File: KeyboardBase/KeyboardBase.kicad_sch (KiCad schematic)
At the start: 2 parts, among them J101 Conn_01x07, U101 74HC00

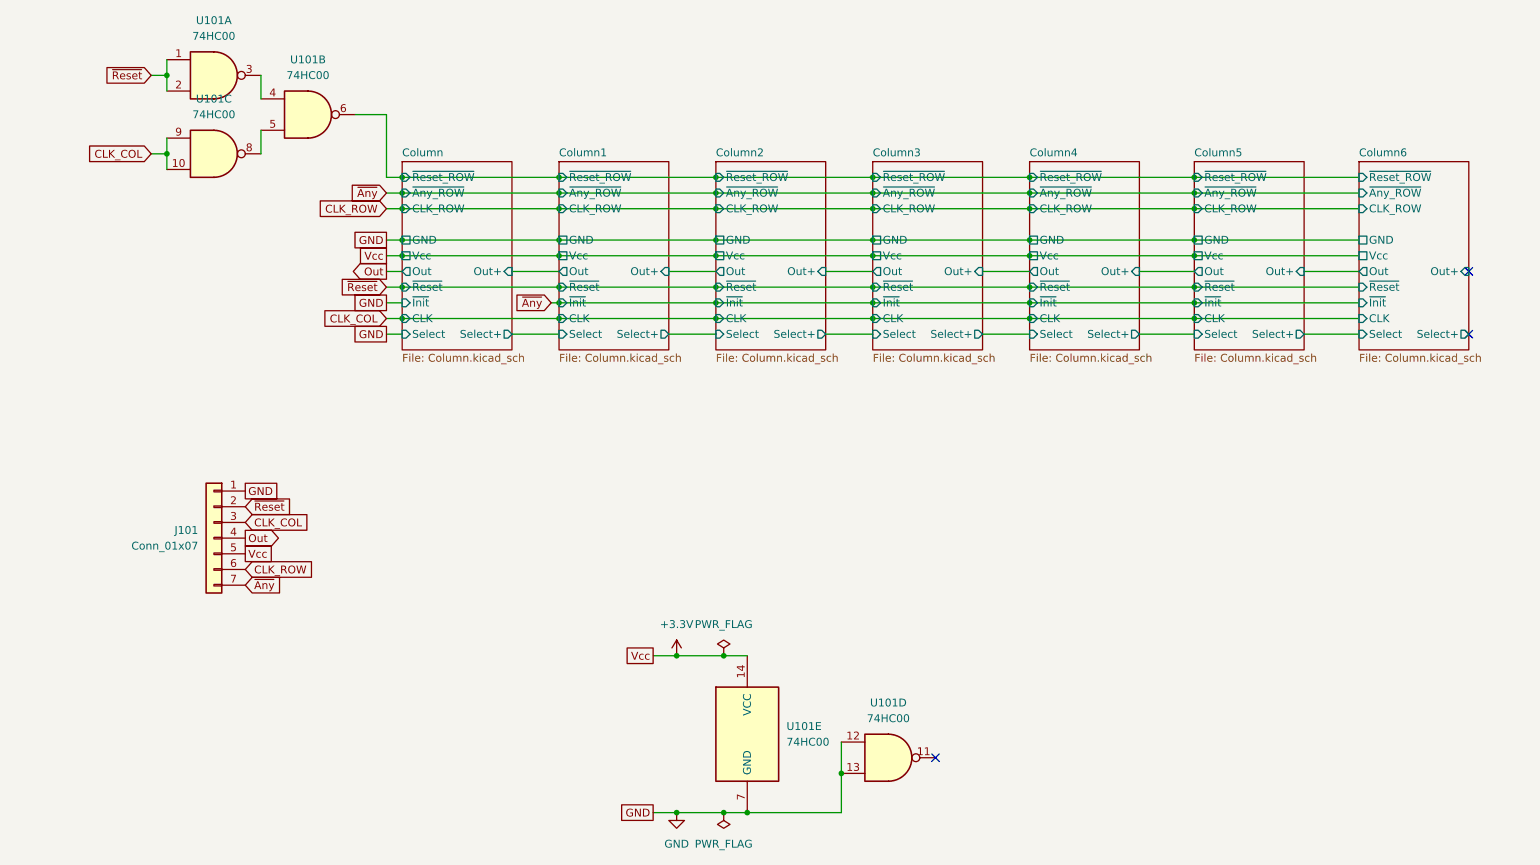
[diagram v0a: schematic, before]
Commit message: fix circuit
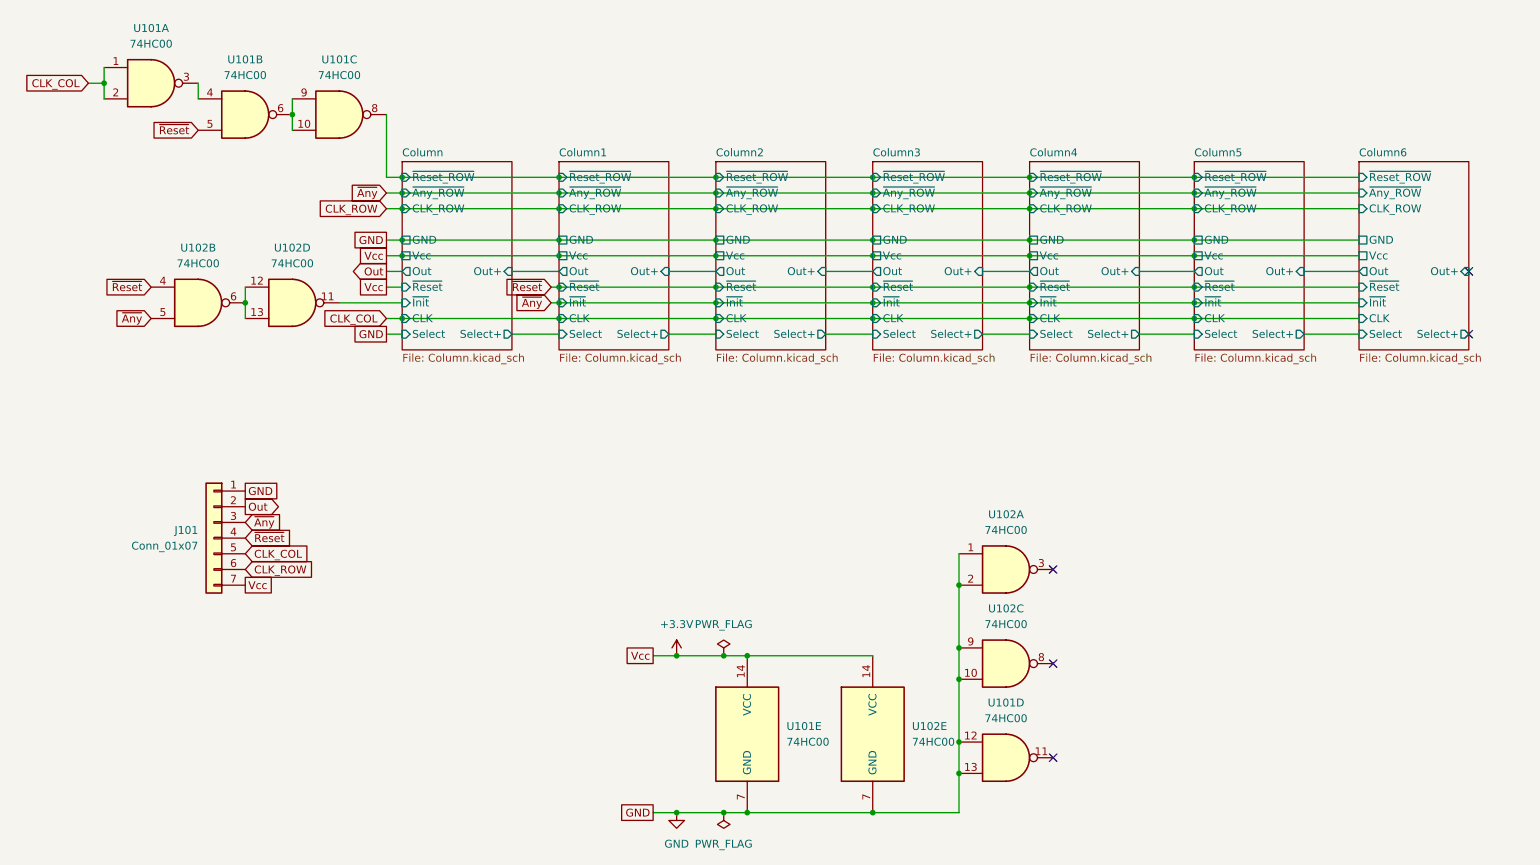
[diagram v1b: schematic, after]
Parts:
- added U102: 74HC00, Package_DFN_QFN:WQFN-14-1EP_2.5x2.5mm_P0.5mm_EP1.45x1.45mm, symbol 74xx:74HC00
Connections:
- net +3.3V: now also J101.7 (Pin_7), U102.14 (VCC); no longer J101.5 (Pin_5)
- net CLK_COL: now also J101.5 (Pin_5), U101.1, U101.2; no longer J101.3 (Pin_3), U101.10, U101.9
- net Column/~{Reset_ROW}: now also U101.8; no longer U101.6
- net GND: now also U102.1, U102.10, U102.2, U102.7 (GND), U102.9
- net Out: now also J101.2 (Pin_2); no longer J101.4 (Pin_4)
- net ~{Any}: now also J101.3 (Pin_3), U102.5; no longer J101.7 (Pin_7)
- net ~{Reset}: now also J101.4 (Pin_4), U101.5, U102.4; no longer J101.2 (Pin_2), U101.1, U101.2
- net at U101.4: now also U101.3; no longer U101.3
- new net: U101.10, U101.6, U101.9
- new net: U102.12, U102.13, U102.6
- new net Column/~{Init}: U102.11
- no-connect marks 3 -> 5
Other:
- moved on the sheet: U101A, U101B, U101C, U101D
